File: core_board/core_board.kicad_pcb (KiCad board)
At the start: 2 copper layers, 81.3 x 101.6 mm, 111 parts, among them J1 Molex_Megafit_02, J10 Conn_01x04_Pin, J11 Conn_01x02_Pin, J12 Conn_01x02_Pin, J13 Conn_01x03_Pin, J14 Conn_01x02_Pin, J15 Conn_01x02_Pin, J16 Conn_01x03_Pin, J2 RJ45_LED_Shielded, J3 Conn_01x02_Pin, J4Serv1 Conn_01x04_Pin, J5 Conn_01x04_Pin, J6 Conn_01x02_Pin, J8 Conn_01x04_Pin, J9 Conn_01x02_Pin, Q1 TPC8132_LQS, Q18 BSS138, Q19 BSS138, Q2 BSS138, Q20 BSS138, Q21 BSS138, Q3 BSS138, Q4 BSS138, Q5 BSS138, Q6 BSS138, Q7 BSS138, SW1 SW_Push, SW2 SW_Push, SW3 SW_Push, SW4 SW_Push, U1 AP63301WU7, U4 BD9G401EFJ-E2

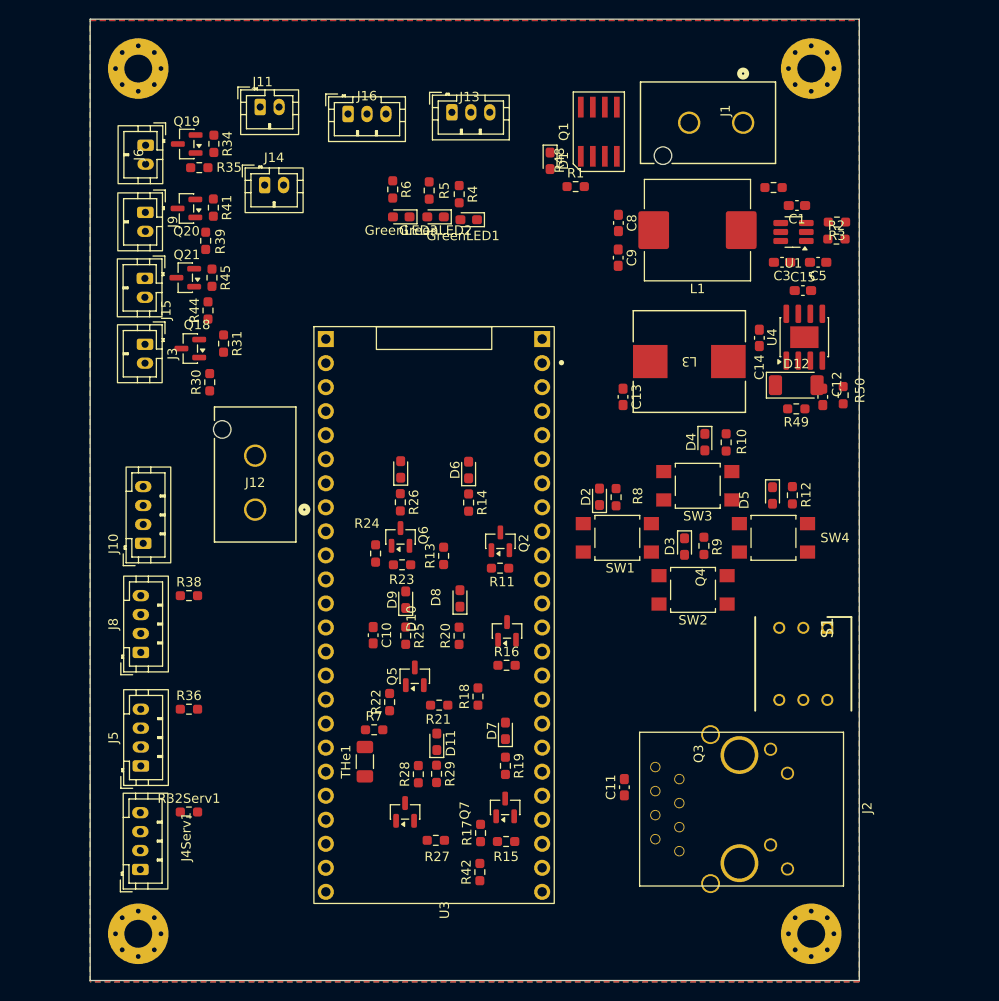
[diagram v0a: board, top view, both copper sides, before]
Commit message: Add new layout
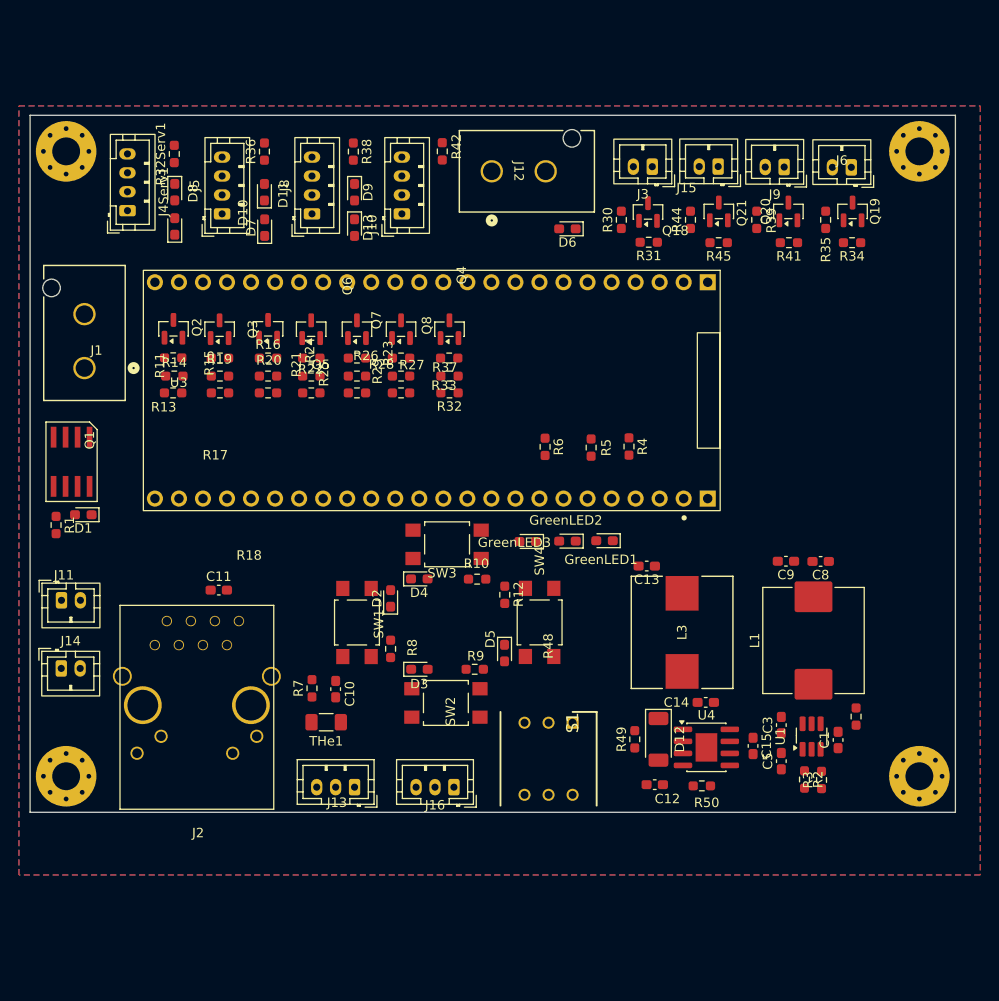
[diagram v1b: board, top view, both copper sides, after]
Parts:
- added D13: Blue, LED_SMD:LED_0603_1608Metric_Pad1.05x0.95mm_HandSolder, F.Cu at (137.2, 65.2)
- added Q8: BSS138, Package_TO_SOT_SMD:SOT-23, F.Cu at (147.2, 75.9)
- added R32: 10k, Resistor_SMD:R_0603_1608Metric_Pad0.98x0.95mm_HandSolder, F.Cu at (147.2, 82.7)
- added R33: 100, Resistor_SMD:R_0603_1608Metric_Pad0.98x0.95mm_HandSolder, F.Cu at (147.2, 80.9)
- added R37: 1k, Resistor_SMD:R_0603_1608Metric_Pad0.98x0.95mm_HandSolder, F.Cu at (147.2, 79.0)
- moved U7 83.0 mm to (106.7, 57.1), turned to -90 degrees
- moved U8 83.0 mm to (196.8, 57.1), turned to -90 degrees
- moved U6 80.5 mm to (106.7, 123.2), turned to -90 degrees
- moved R42 76.3 mm to (146.4, 57.1)
- moved U5 75.7 mm to (196.8, 123.2), turned to -90 degrees
- moved J6 74.6 mm to (189.7, 58.8), turned to 180 degrees
- moved J1 74.3 mm to (108.6, 80.1), turned to 0 degrees
- moved J13 72.1 mm to (137.2, 124.3), turned to 180 degrees
- moved J16 72.0 mm to (147.7, 124.3), turned to 180 degrees
- moved Q19 70.7 mm to (189.8, 63.5), turned to 90 degrees
- moved J2 70.2 mm to (120.6, 128.7), turned to 0 degrees
- moved J4Serv1 69.6 mm to (113.2, 63.4)
- moved R32Serv1 69.6 mm to (118.1, 57.4), turned to 90 degrees
- moved R34 68.3 mm to (189.7, 66.8), turned to 180 degrees
- moved J9 67.7 mm to (182.6, 58.8), turned to 180 degrees
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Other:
- board size 81.3 x 101.6 mm -> 97.8 x 73.7 mm
